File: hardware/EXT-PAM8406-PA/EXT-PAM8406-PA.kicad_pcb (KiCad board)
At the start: 2 copper layers, 10.1 x 50.8 mm, 18 parts, among them J1 EXT, J2 JST-XH 2.54mm 2P, J3 JST-XH 2.54mm 2P, J4 PicoBlade_2P_P1.25mm_Horizont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, J6 PicoBlade_2P_P1.25mm_Horizont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, U1 PAM8406D

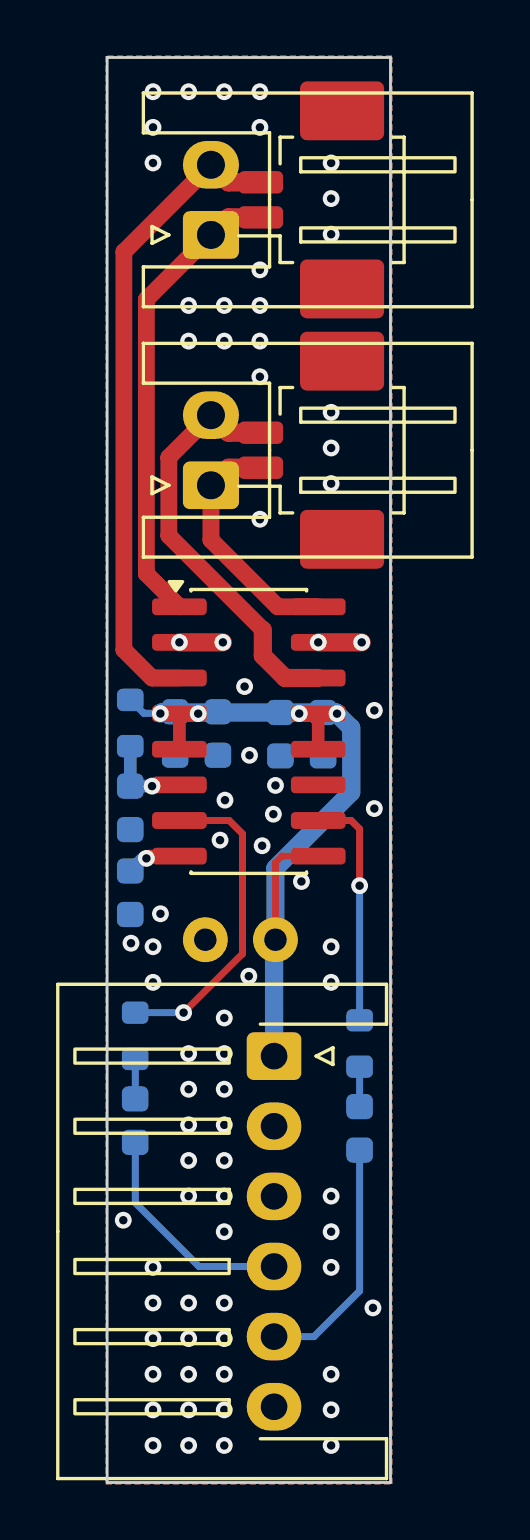
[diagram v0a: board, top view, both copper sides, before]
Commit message: hardware: add misc project files
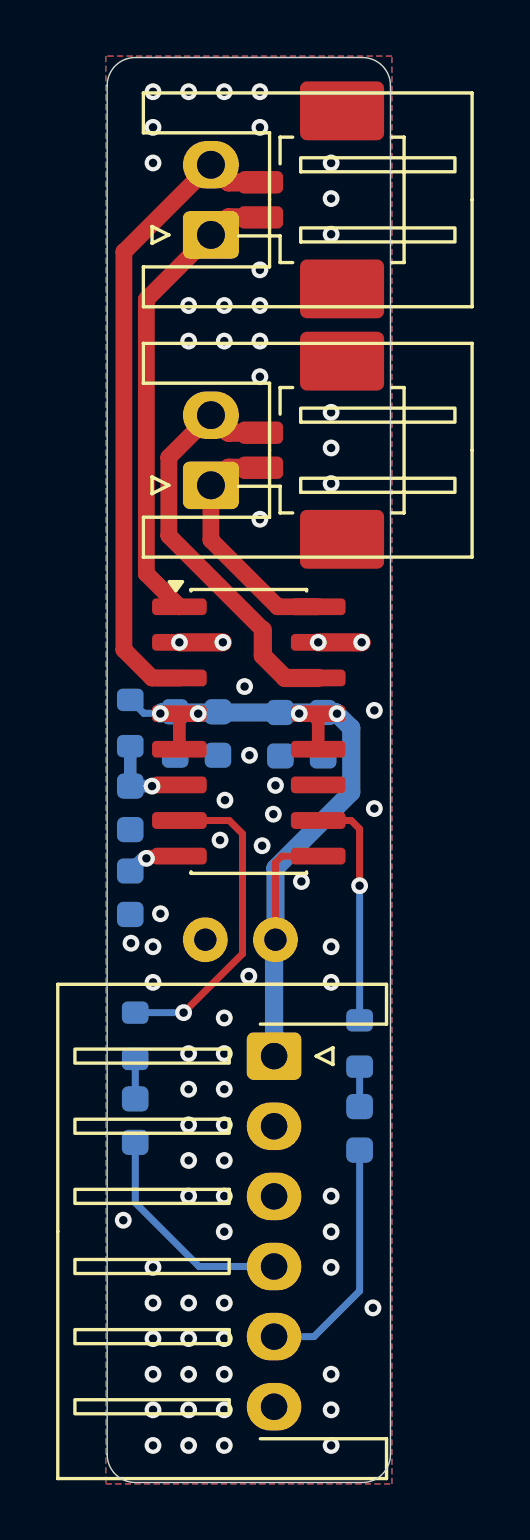
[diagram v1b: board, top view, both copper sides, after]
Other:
- outline, holes or cut-outs redrawn
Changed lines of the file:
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@@
 		)
 	)
-	(gr_rect
-		(start 137.5 73.875)
-		(end 147.6 124.675)
+	(gr_line
+		(start 147.6 74.875)
+		(end 147.6 123.675)
 		(stroke
-			(width 0.1)
+			(width 0.05)
 			(type default)
 		)
-		(fill no)
 		(layer "Edge.Cuts")
 	)
+	(gr_arc
+		(start 146.6 73.875)
+		(mid 147.307107 74.167893)
+		(end 147.6 74.875)
+		(stroke
+			(width 0.05)
+			(type default)
+		)
+		(layer "Edge.Cuts")
+	)
+	(gr_arc
+		(start 138.5 124.675)
+		(mid 137.792893 124.382107)
+		(end 137.5 123.675)
+		(stroke
+			(width 0.05)
+			(type default)
+		)
+		(layer "Edge.Cuts")
+	)
+	(gr_line
+		(start 146.6 124.675)
+		(end 138.5 124.675)
+		(stroke
+			(width 0.05)
+			(type default)
+		)
+		(layer "Edge.Cuts")
+	)
+	(gr_arc
+		(start 147.6 123.675)
+		(mid 147.307107 124.382107)
+		(end 146.6 124.675)
+		(stroke
+			(width 0.05)
+			(type default)
+		)
+		(layer "Edge.Cuts")
+	)
+	(gr_line
+		(start 138.5 73.875)
+		(end 146.6 73.875)
+		(stroke
+			(width 0.05)
+			(type default)
+		)
+		(layer "Edge.Cuts")
+	)
+	(gr_arc
+		(start 137.5 74.875)
+		(mid 137.792893 74.167893)
+		(end 138.5 73.875)
+		(stroke
+			(width 0.05)
+			(type default)
+		)
+		(layer "Edge.Cuts")
+	)
+	(gr_line
+		(start 137.5 123.675)
+		(end 137.5 74.875)
+		(stroke
+			(width 0.05)
+			(type default)
+		)
+		(layer "Edge.Cuts")
+	)
